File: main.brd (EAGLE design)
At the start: 25.1 x 24.8 mm, 32 parts, among them IC1 ATTINY13A-SSH, T1A 2N4401, T1B NPN, T2A 2N4401, T2B NPN

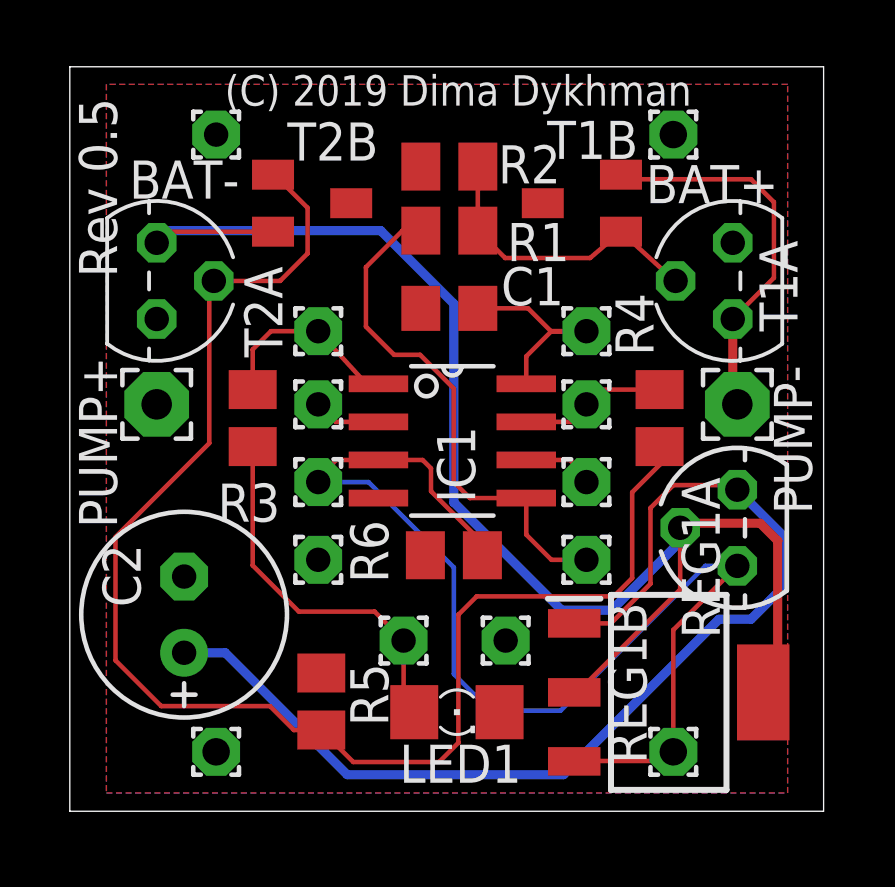
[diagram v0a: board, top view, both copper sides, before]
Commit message: code updates
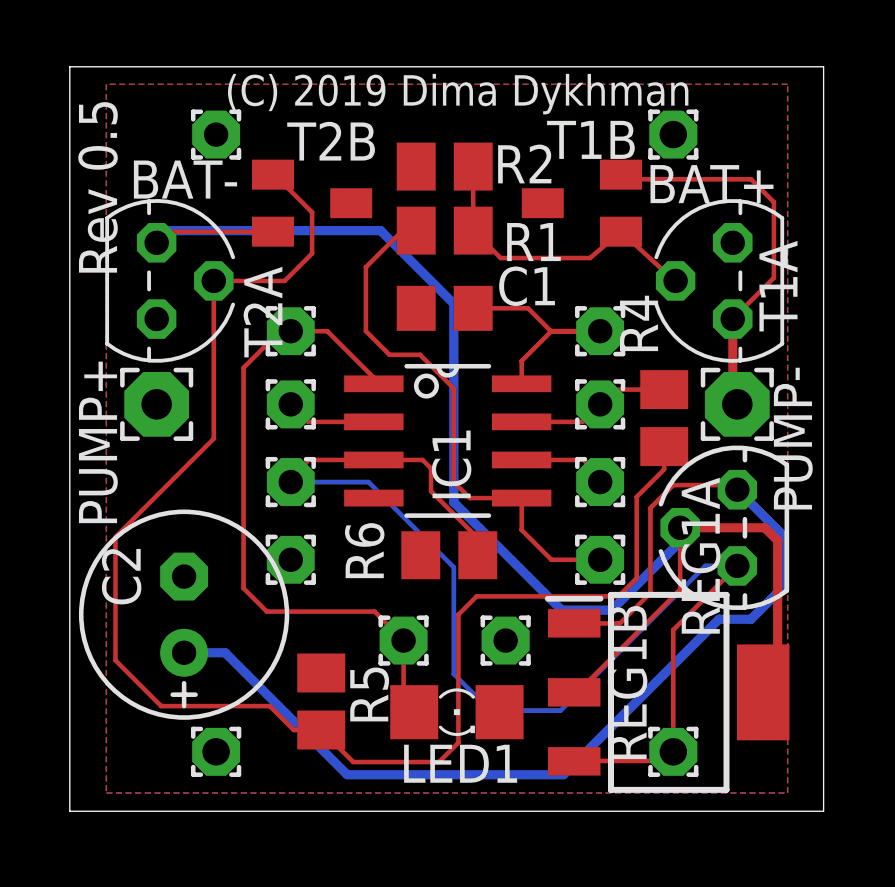
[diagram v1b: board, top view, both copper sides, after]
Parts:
- removed R3: 120, resistor:M0805
- moved PAD10 0.91 mm to (7.98, 16.5)
- moved PAD7 0.91 mm to (7.98, 8.84)
- moved PAD8 0.91 mm to (7.98, 11.4)
- moved PAD9 0.91 mm to (7.98, 14.0)
- moved PAD3 0.46 mm to (18.3, 16.5)
- moved PAD4 0.46 mm to (18.3, 14.0)
- moved PAD5 0.46 mm to (18.3, 8.84)
- moved PAD6 0.46 mm to (18.3, 11.4)
- moved C1 0.15 mm to (13.1, 17.2)
- moved IC1 0.15 mm to (13.2, 12.8)
- moved R1 0.15 mm to (13.1, 19.8)
- moved R2 0.15 mm to (13.1, 21.9)
- moved R4 0.15 mm to (20.4, 13.6)
- moved R6 0.15 mm to (13.3, 8.99)
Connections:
- removed net N$3: LED1.A, PAD1.1, R3.2
- net LED: now also LED1.A, PAD1.1; no longer R3.1
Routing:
- net LED: track 6.55 -> 21.6 mm
- net N$3: track 12.6 -> 0.00 mm
- net SENSOR-: track 39.6 -> 41.3 mm
- net VCC: track 7.21 -> 8.34 mm
- net UART_TX: track 2.25 -> 3.01 mm
- net SENSOR+: track 2.38 -> 2.99 mm

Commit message: rev 0.6
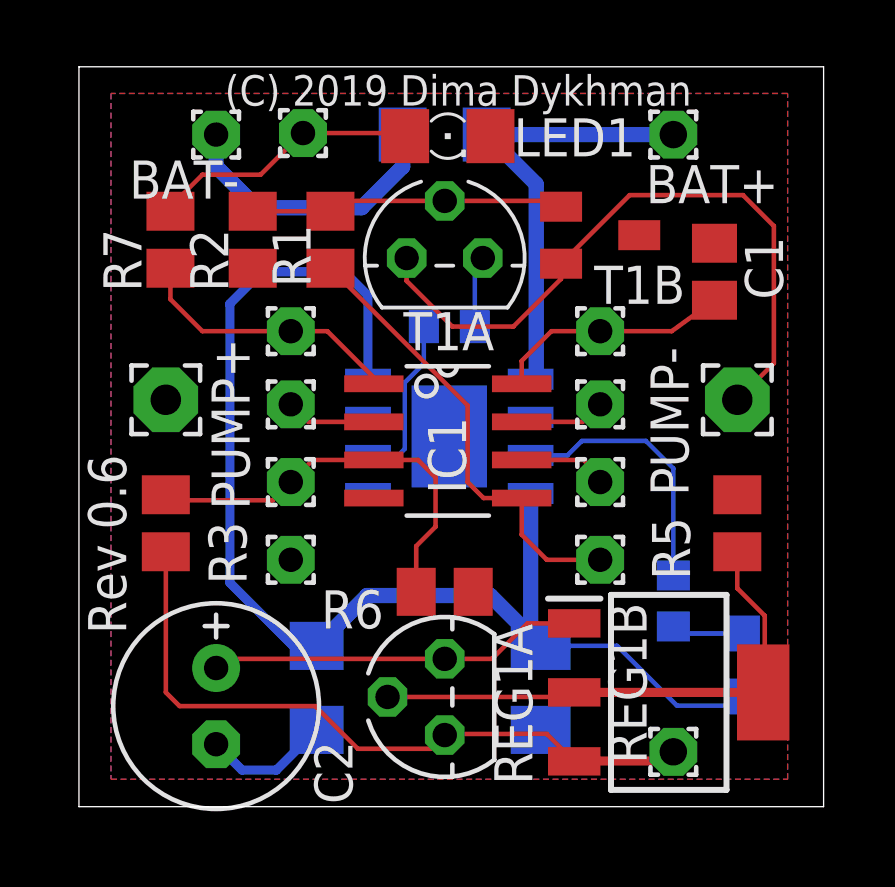
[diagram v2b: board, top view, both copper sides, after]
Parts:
- removed IN-: 5V, wirepad:1,6/0,9
- removed PAD2: (no value), wirepad:1,6/0,8
- removed T2A: 2N4401, transistor:TO92
- removed T2B: NPN, semicon-smd-ipc:SOT23W
- added C3, C4: 10uF, rcl:C3216
- added IC2: TP4056-42-ESOP8, 1EDI60I12AF:SOIC127P600X175-9N
- added LED2: (no value), led:SML0805
- added R3: 10k, resistor:M0805
- added R7: 510, resistor:M0805
- added R8: 10k, rcl:R0603
- added R9: 1.2k, rcl:R0603
- R4: value 510 -> R400; device resistor:M0805 -> resistor:M1206
- moved LED1 19.2 mm to (13.2, 23.0)
- moved PAD1 17.2 mm to (8.38, 23.1)
- moved R5 15.1 mm to (22.9, 10.1)
- moved REG1A 11.3 mm to (13.1, 4.27)
- moved R4 9.89 mm to (16.3, 4.57), flipped to the bottom, turned to 90 degrees
- moved T1A 9.63 mm to (13.1, 18.9), turned to 0 degrees
- moved C1 9.07 mm to (22.1, 18.4), turned to 90 degrees
- moved R2 6.85 mm to (6.71, 19.5), turned to 90 degrees
- moved R1 3.82 mm to (9.30, 19.5), turned to 270 degrees
- moved C2 3.23 mm to (5.49, 3.96), turned to 270 degrees
- moved T1B 1.23 mm to (18.3, 19.7), turned to 270 degrees
- moved R6 1.23 mm to (13.1, 7.77), turned to 0 degrees
- moved PUMP+ 0.34 mm to (3.81, 14.2)
- moved PUMP- 0.15 mm to (22.9, 14.2)
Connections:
- new net N$11: IC2.2, R9.1
- new net N$3: IN+.1, R3.2, REG1A.1, REG1B.3
- new net N$6: LED1.A, PAD1.1, R7.2
- new net N$7: BAT+.1, C4.1, IC2.5
- new net N$8: IC2.7, R8.2
- new net N$9: LED2.C, R8.1
- net GND: now also C3.2, C4.2, R9.2; no longer IN-.1, PAD2.1, T2A.1, T2B.3
- net LED: now also R7.1; no longer LED1.A, PAD1.1
- net N$4: now also C3.1, IC2.4, IC2.8, LED2.A; no longer R5.2, T2A.2, T2B.1
- net N$5: now also R5.2; no longer T2A.3, T2B.2
- net SENSOR-: now also R3.1; no longer IN+.1, REG1A.1, REG1B.3
- net SOLAR: no longer R4.1
- net VCC: now also R4.1; no longer BAT+.1
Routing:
- net N$5: track 48.1 -> 17.8 mm
- net SENSOR-: track 41.3 -> 13.9 mm
- net SOLAR_PANEL+: track 37.2 -> 12.6 mm
- net N$3: track 0.00 -> 23.1 mm
- net GND: track 0.00 -> 16.2 mm
- net N$7: track 0.00 -> 15.1 mm
- net LED: track 21.6 -> 9.10 mm
- net N$2: track 12.9 -> 22.5 mm
- net N$6: track 0.00 -> 9.03 mm
- net N$8: track 0.00 -> 8.90 mm
- net N$4: track 49.4 -> 43.0 mm
- net N$11: track 0.00 -> 5.66 mm
- net PUMP: track 17.7 -> 15.2 mm
- net N$9: track 0.00 -> 2.38 mm
- net SOLAR: track 5.20 -> 2.86 mm
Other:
- board size 25.1 x 24.8 mm -> 24.8 x 24.7 mm
- board text added: "Rev 0.6"
- board text removed: "Rev 0.5"
